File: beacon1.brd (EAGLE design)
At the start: 160 x 100 mm, 89 parts, among them IC1 NCP1117ST50T3G, IC6 LP2985-33DBVR, IC7 LMV358IDGKR, Q4 220mA/50V/3.5Ω, Q5 220mA/50V/3.5Ω, Q6 220mA/50V/3.5Ω, Q7 220mA/50V/3.5Ω, T1 FDN340P, U1 FGPMMOPA6H, U2 MIC5225-3.3, Y1 CSTCE16M0V53-R0 16MHZ

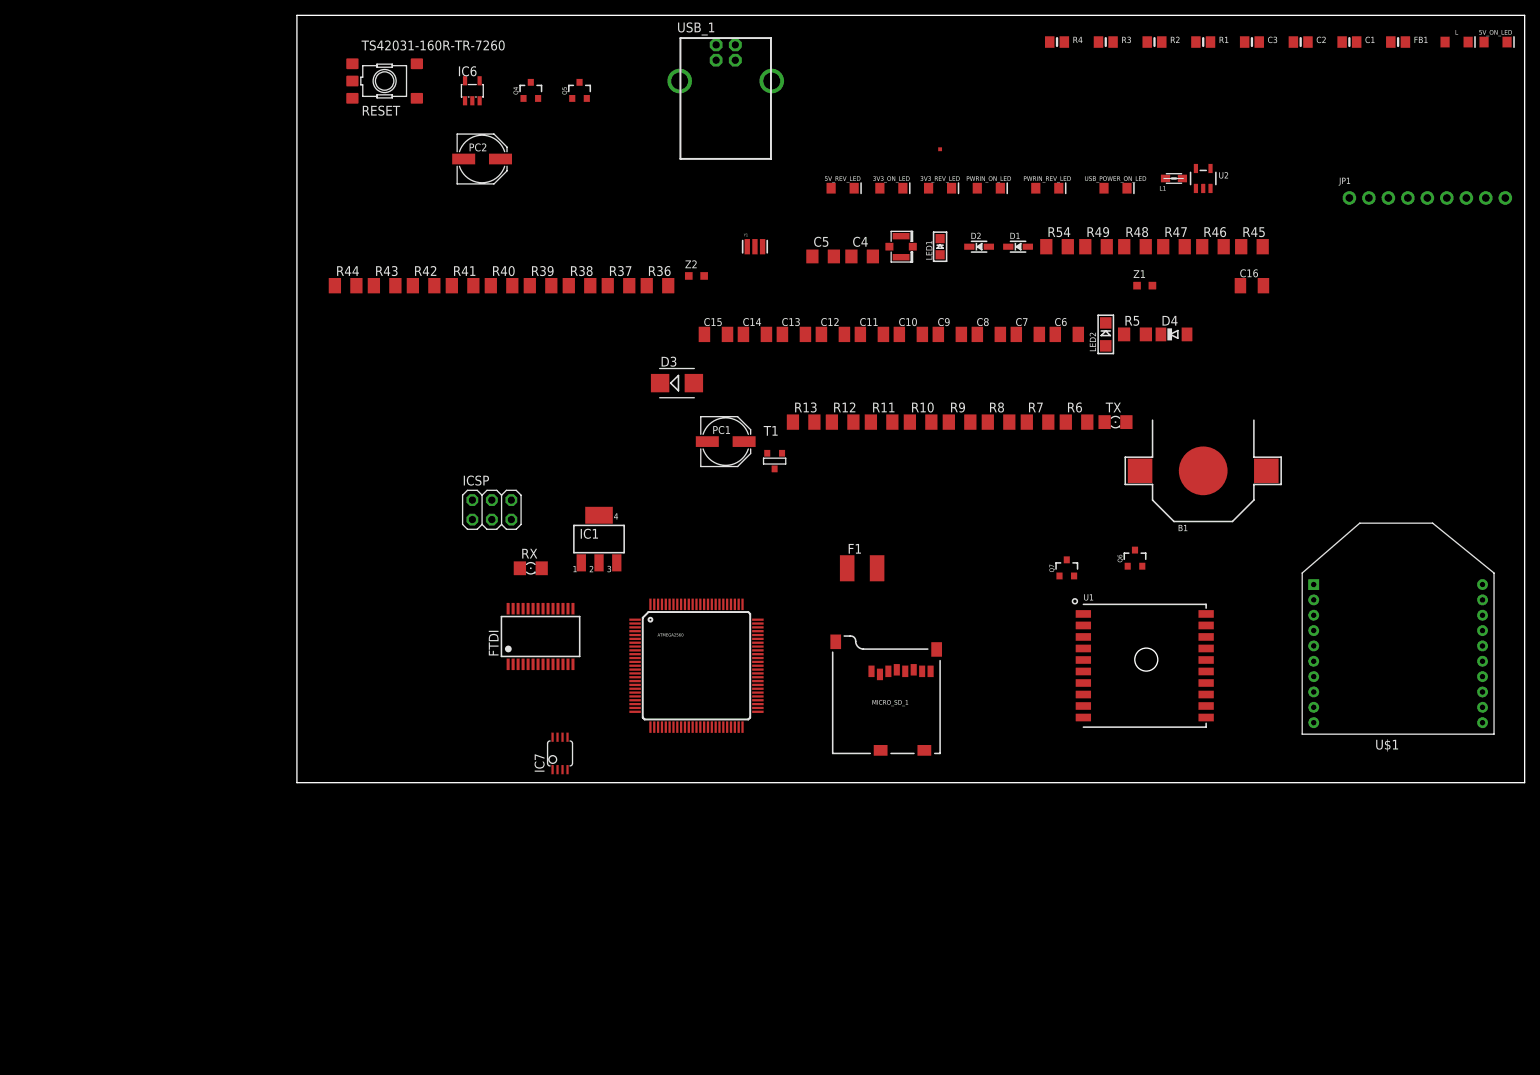
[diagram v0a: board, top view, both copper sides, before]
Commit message: added bluetooth chip and condensed layout somewhat, still not routed
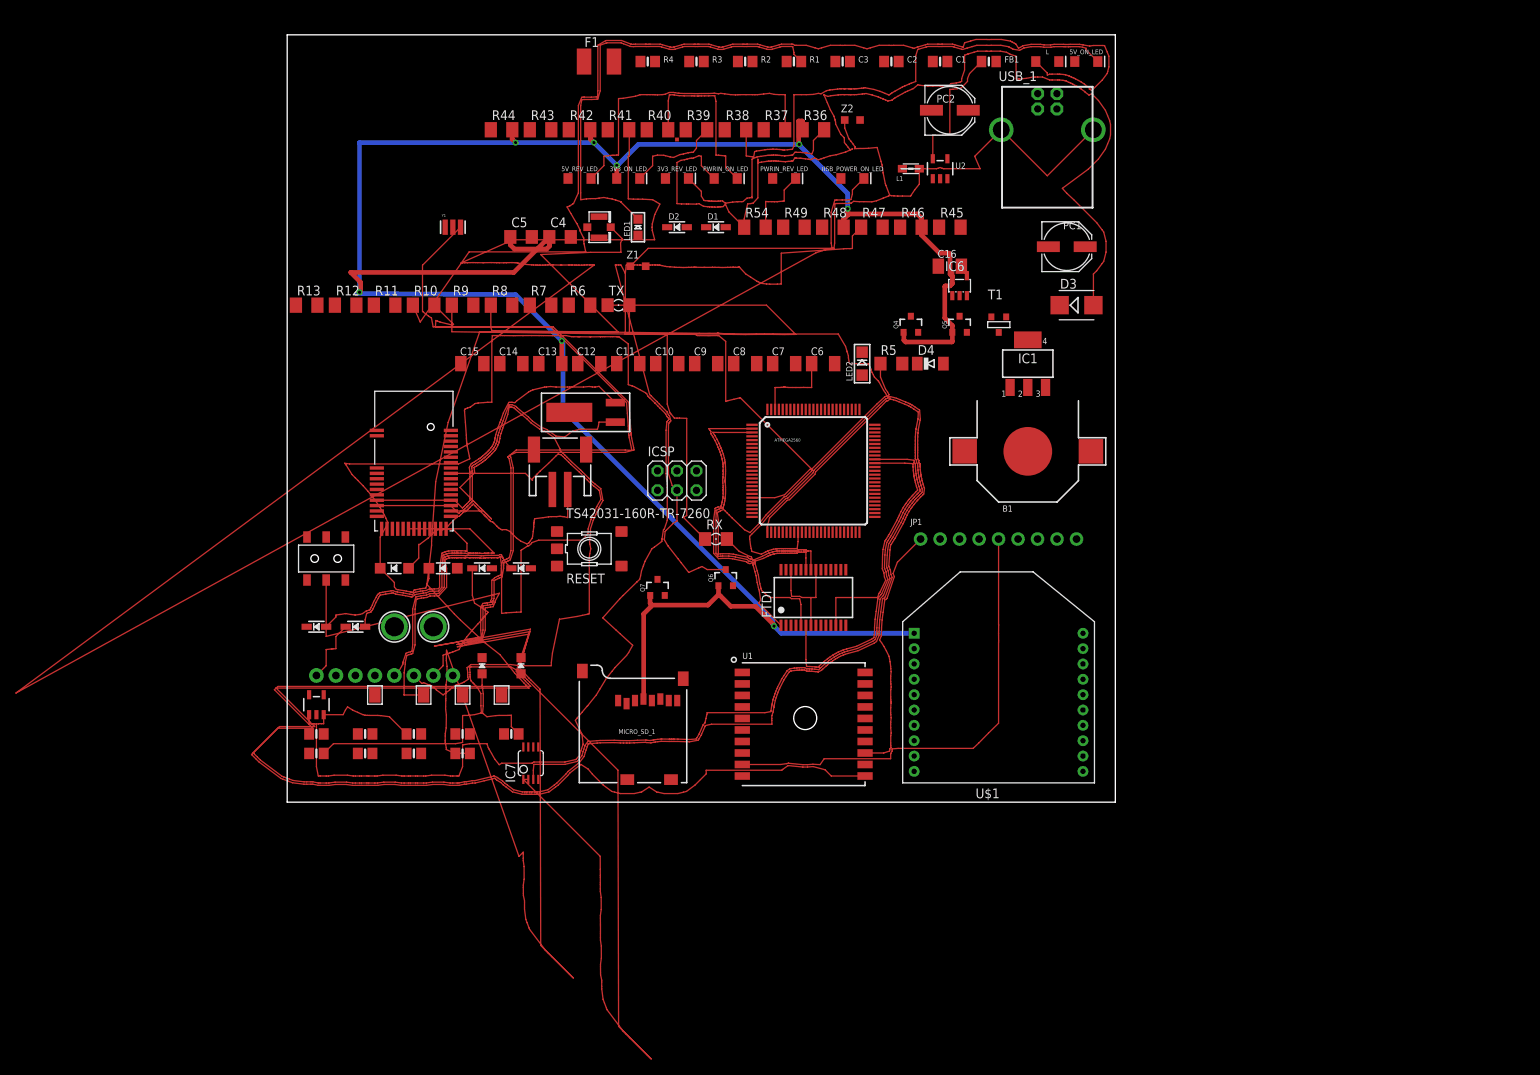
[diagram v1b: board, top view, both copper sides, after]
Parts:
- added C17, C18: 1uF, microbuilder:0805-NO
- added C19, C20: 10uF, microbuilder:0805-NO
- added D10, D11, D8, D9: 1n4148, microbuilder:SOD-323
- added D12, D7: MBR120, microbuilder:SOD-123
- added D5: RED, microbuilder:CHIPLED_0805_NOOUTLINE
- added D6: GREEN, microbuilder:CHIPLED_0805_NOOUTLINE
- added JP2: (no value), microbuilder:1X08_ROUND_76
- added R14, R15: 1K, microbuilder:0805-NO
- added R16, R17: 100K, microbuilder:0805-NO
- added R18: 2K, microbuilder:0805-NO
- added SW1: EG1319, microbuilder:EG1390
- added TP1: SWCLK, microbuilder:PAD-1.5X2.0
- added TP2: SWDIO, microbuilder:PAD-1.5X2.0
- added TP3, VTREF: FCTRST, microbuilder:PAD-1.5X2.0
- added U$31, U$32: MOUNTINGHOLE2.5, microbuilder:MOUNTINGHOLE_2.5_PLATED
- added U3: (no value), microbuilder:BLE_MODULE_RAYTAC_MDBT40
- added U4: MIC5225-3.3, microbuilder:SOT23-5
- added X1: JST 2PH, microbuilder:JSTPH2
- added Y2: 32.768kHz (535-9166-2-ND), microbuilder:CRYSTAL_CYL_2X6MM_SMT
- FB1: device microbuilder:0805-NO -> microbuilder:0805-NO@1
- moved F1 74.4 mm to (39.4, 94.0)
- moved JP1 71.4 mm to (91.4, 31.8)
- moved IC6 68.4 mm to (86.4, 64.8)
- moved R11 66.5 mm to (11.4, 62.2)
- moved R12 66.5 mm to (6.35, 62.2)
- moved R13 66.5 mm to (1.27, 62.2)
- moved TX 66.5 mm to (41.9, 62.2)
- moved R10 66.5 mm to (16.5, 62.2)
- moved R6 66.5 mm to (36.8, 62.2)
- moved R7 66.5 mm to (31.8, 62.2)
- moved R8 66.5 mm to (26.7, 62.2)
- moved R9 66.5 mm to (21.6, 62.2)
- moved RESET 66.5 mm to (38.1, 30.5)
- moved Z1 66.1 mm to (44.5, 67.3)
- moved PC2 61.3 mm to (85.1, 87.6)
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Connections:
- new net CONNECTED_LED: R15.1, U3.39
- new net CTS_3V: D8.A, R16.1, U3.28
- new net CTS_5V: D8.C, JP2.7
- new net DCC: U3.15
- new net DEC2: U3.41
- new net DFU_3V: D11.A, U3.24
- new net DFU_5V: D11.C, JP2.1
- new net FCTRYRST_3V: TP3.P$1, U3.34
- new net MODE_3V: D10.A, U3.18
- new net MODE_5V: D10.C, JP2.8, R18.1
- new net MODE_LED: R14.1, U3.38
- new net N$15: D5.A, R14.2
- new net N$16: D6.A, R15.2
- new net N$17: U3.9, Y2.1
- new net N$18: U3.10, Y2.2
- new net N$19: R18.2, SW1.P2
- new net N$21: C19.1, D12.C, D7.C, U4.1, U4.3
- new net RTS_O: JP2.3, U3.26
- new net RXD_3V: D9.A, R17.1, U3.29
- new net RXD_5V: D9.C, JP2.5
- new net SWCLK: TP1.P$1, U3.36
- new net SWDIO/RST_3V: TP2.P$1, U3.35
- new net TX_O: JP2.6, U3.27
- new net VBAT: D7.A, X1.2
- net 3.3V: now also C17.1, C18.1, C20.1, R16.2, R17.2, SW1.O2, U3.14, U3.3, U4.5, VTREF.P$1
- net GND: now also C17.2, C18.2, C19.2, C20.2, D5.C, D6.C, JP2.2, SW1.S2, U3.1, U3.13, U3.16, U3.2, U3.25, U3.42, U4.2, X1.1
- net VIN: now also D12.A, JP2.4
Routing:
- net XTAL1: track 0.00 -> 342.5 mm
- net 3V3: track 0.00 -> 312.1 mm, vias 0 -> 8
- net N$14: track 0.00 -> 288.4 mm
- net N$4: track 0.00 -> 236.6 mm
- net N$21: track 0.00 -> 207.1 mm
- net L13: track 0.00 -> 204.9 mm
- net N$19: track 0.00 -> 162.8 mm
- net SCK: track 0.00 -> 143.4 mm
- net N$7: track 0.00 -> 142.9 mm
- net PWRIN: track 0.00 -> 131.0 mm
- net PB7: track 0.00 -> 115.3 mm
- net TXL: track 0.00 -> 93.0 mm
- net USHIELD: track 0.00 -> 92.6 mm
- net TX_O: track 0.00 -> 88.9 mm
- net FCTRYRST_3V: track 0.00 -> 87.8 mm
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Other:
- board size 160 x 100 mm -> 107.9 x 100 mm
